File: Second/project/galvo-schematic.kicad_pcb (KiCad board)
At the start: 2 copper layers, 30.5 x 32 mm, 22 parts, among them J1 0022272031, U1 TL084, U2 MCP4822, X2 JST-XH-03-PIN-ROUND-PAD, X3 JST-XH-03-PIN-ROUND-PAD

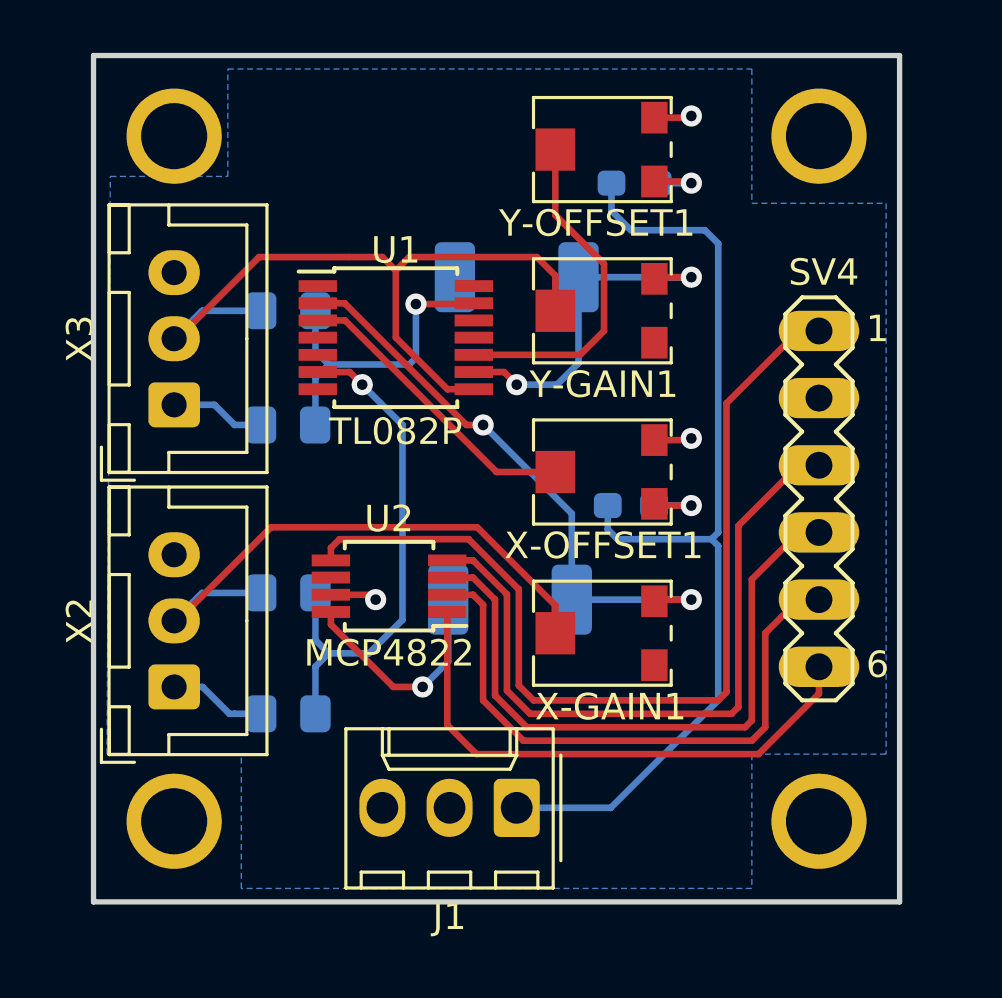
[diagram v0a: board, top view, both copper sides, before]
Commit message: Предварительно закончен второй проект
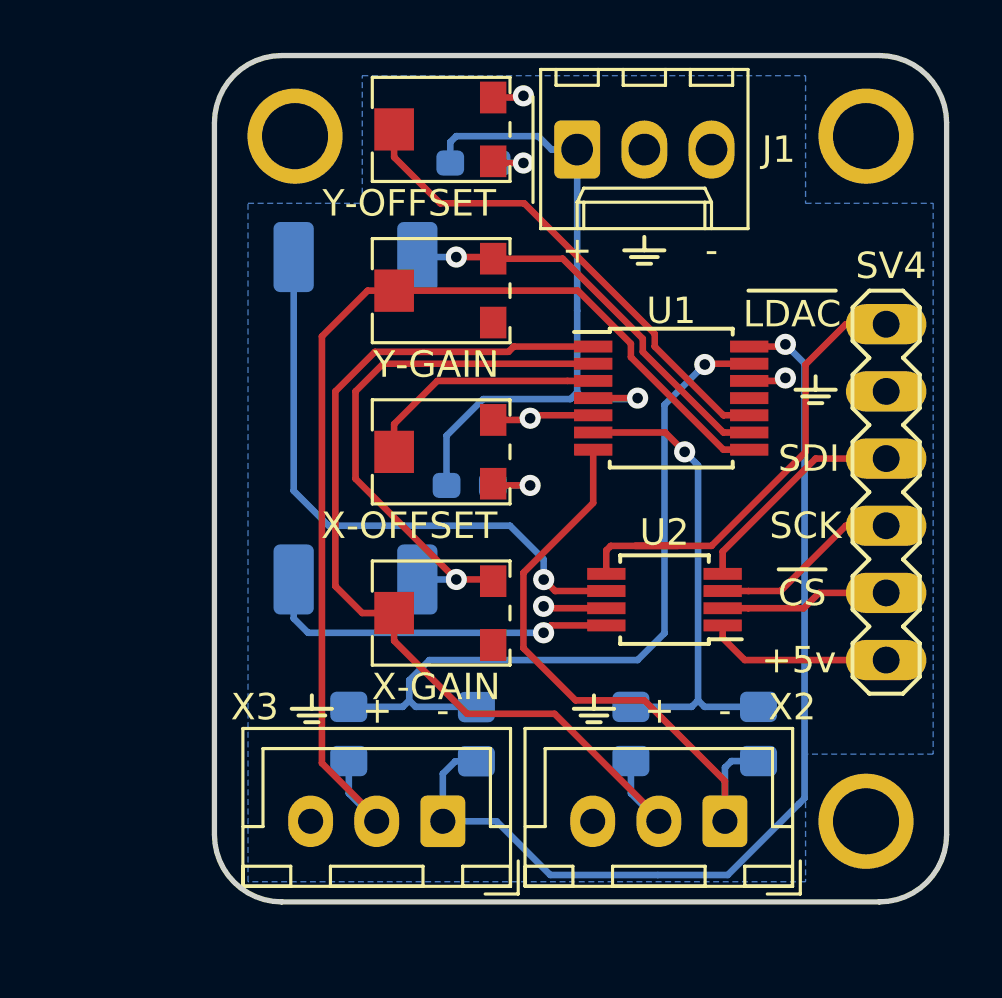
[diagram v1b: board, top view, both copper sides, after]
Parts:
- removed the REF** at (119.9, 84.8)
- removed the REF** at (119.9, 110.7)
- removed the REF** at (144.3, 84.8)
- removed X-GAIN1: 10k, galvo-schematic:Potentiometer_Murata_PVS3_Vertical
- added REF**: MountingHole_2.5mm, MountingHole:MountingHole_2.5mm, F.Cu at (124.5, 84.8)
- added REF**: MountingHole_2.5mm, MountingHole:MountingHole_2.5mm, F.Cu at (146.1, 84.8)
- added X-GAIN: 10k, galvo-schematic:Potentiometer_Murata_PVS3_Vertical, F.Cu at (130.0, 102.9)
- moved J1 25.0 mm to (135.1, 85.3), turned to 0 degrees
- moved X2 21.4 mm to (140.7, 110.7), turned to 180 degrees
- moved X3 18.7 mm to (130.0, 110.7), turned to 180 degrees
- moved R11 17.8 mm to (142.0, 107.4), turned to 270 degrees
- moved R3 16.2 mm to (126.5, 107.4), turned to 90 degrees
- moved R7 14.0 mm to (137.2, 107.4), turned to 90 degrees
- moved R12 13.7 mm to (131.3, 107.5), turned to 270 degrees
- moved U1 10.7 mm to (138.7, 94.7)
- moved U2 10.4 mm to (138.4, 102.4)
- moved R1 6.14 mm to (126.7, 89.4)
- moved R6 6.14 mm to (131.1, 98.0)
- moved X-OFFSET 6.14 mm to (130.0, 96.8)
- moved Y-GAIN 6.14 mm to (130.0, 90.7)
- moved Y-OFFSET 6.14 mm to (130.0, 84.6)
- moved R2 6.14 mm to (131.2, 85.9)
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- renumbered X-OFFSET1 to X-OFFSET, Y-GAIN1 to Y-GAIN, Y-OFFSET1 to Y-OFFSET
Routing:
- net /ILDAY-15V: track 3.60 -> 37.9 mm, vias 0 -> 1
- net Net-(DAC1-Pad6): track 0.00 -> 22.7 mm, vias 0 -> 1
- net /ILDAX-15V: track 3.71 -> 23.2 mm
- net /SDI: track 26.5 -> 7.72 mm
- net /SCK: track 24.7 -> 6.44 mm
- net /LATCH: track 35.9 -> 17.8 mm
- net /CS: track 22.8 -> 5.66 mm
- net Net-(R12-Pad1): track 12.4 -> 28.7 mm
- net /ILDAX+15V: track 21.9 -> 37.1 mm
- net +5V: track 20.7 -> 6.24 mm
- net /ILDAY+15V: track 27.8 -> 41.6 mm
- net /+V15: track 37.4 -> 26.7 mm, vias 0 -> 1
- net Net-(U1-Pad10): track 12.9 -> 18.8 mm
- net Net-(DAC1-Pad8): track 8.62 -> 13.6 mm
- net GND: track 4.61 -> 8.84 mm, vias 3 -> 4
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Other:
- board size 30.5 x 32 mm -> 27.7 x 32 mm
- board text added: "+"
- board text added: "+5v"
- board text added: "-"
- board text added: "CS"
- board text added: "LDAC"
- board text added: "SCK"
- board text added: "SDI"
